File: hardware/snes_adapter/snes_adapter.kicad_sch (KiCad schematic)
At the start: 4 parts, among them J1 CART SLOT TOP ROW, J2 CART SLOT BOTTOM ROW, J3 SNES_Slot

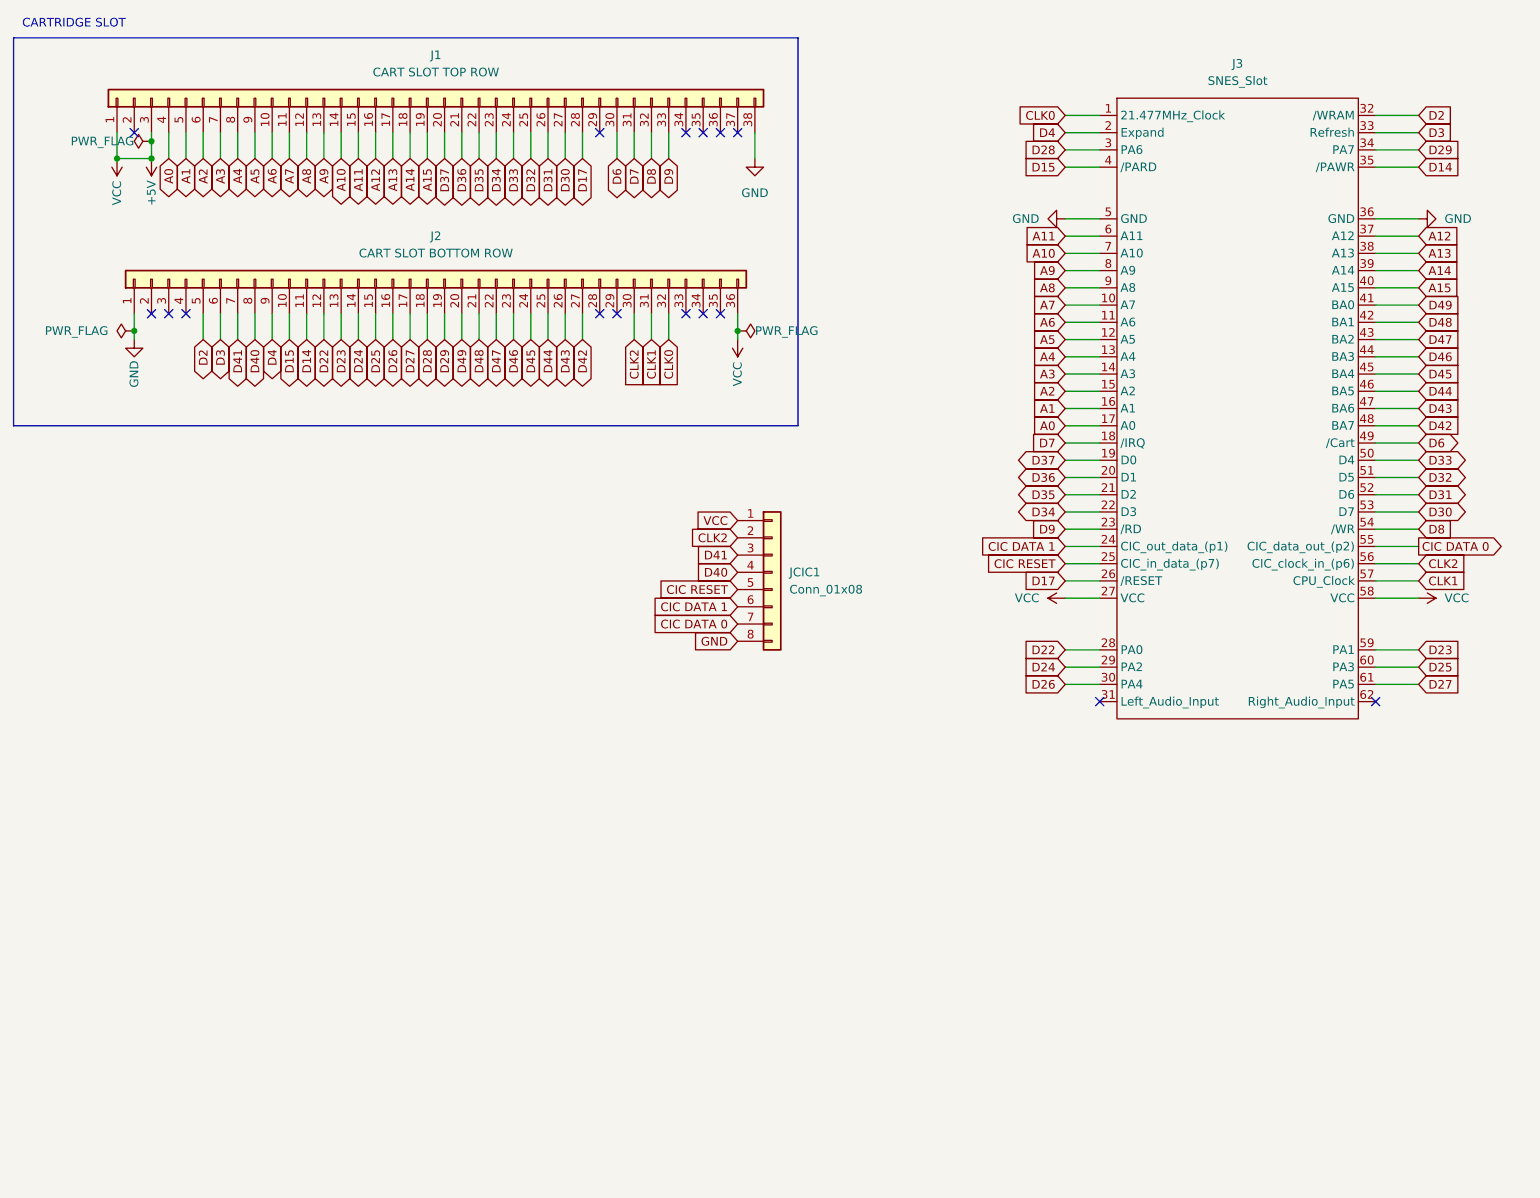
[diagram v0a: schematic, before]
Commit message: Move SNES updates to clean branch
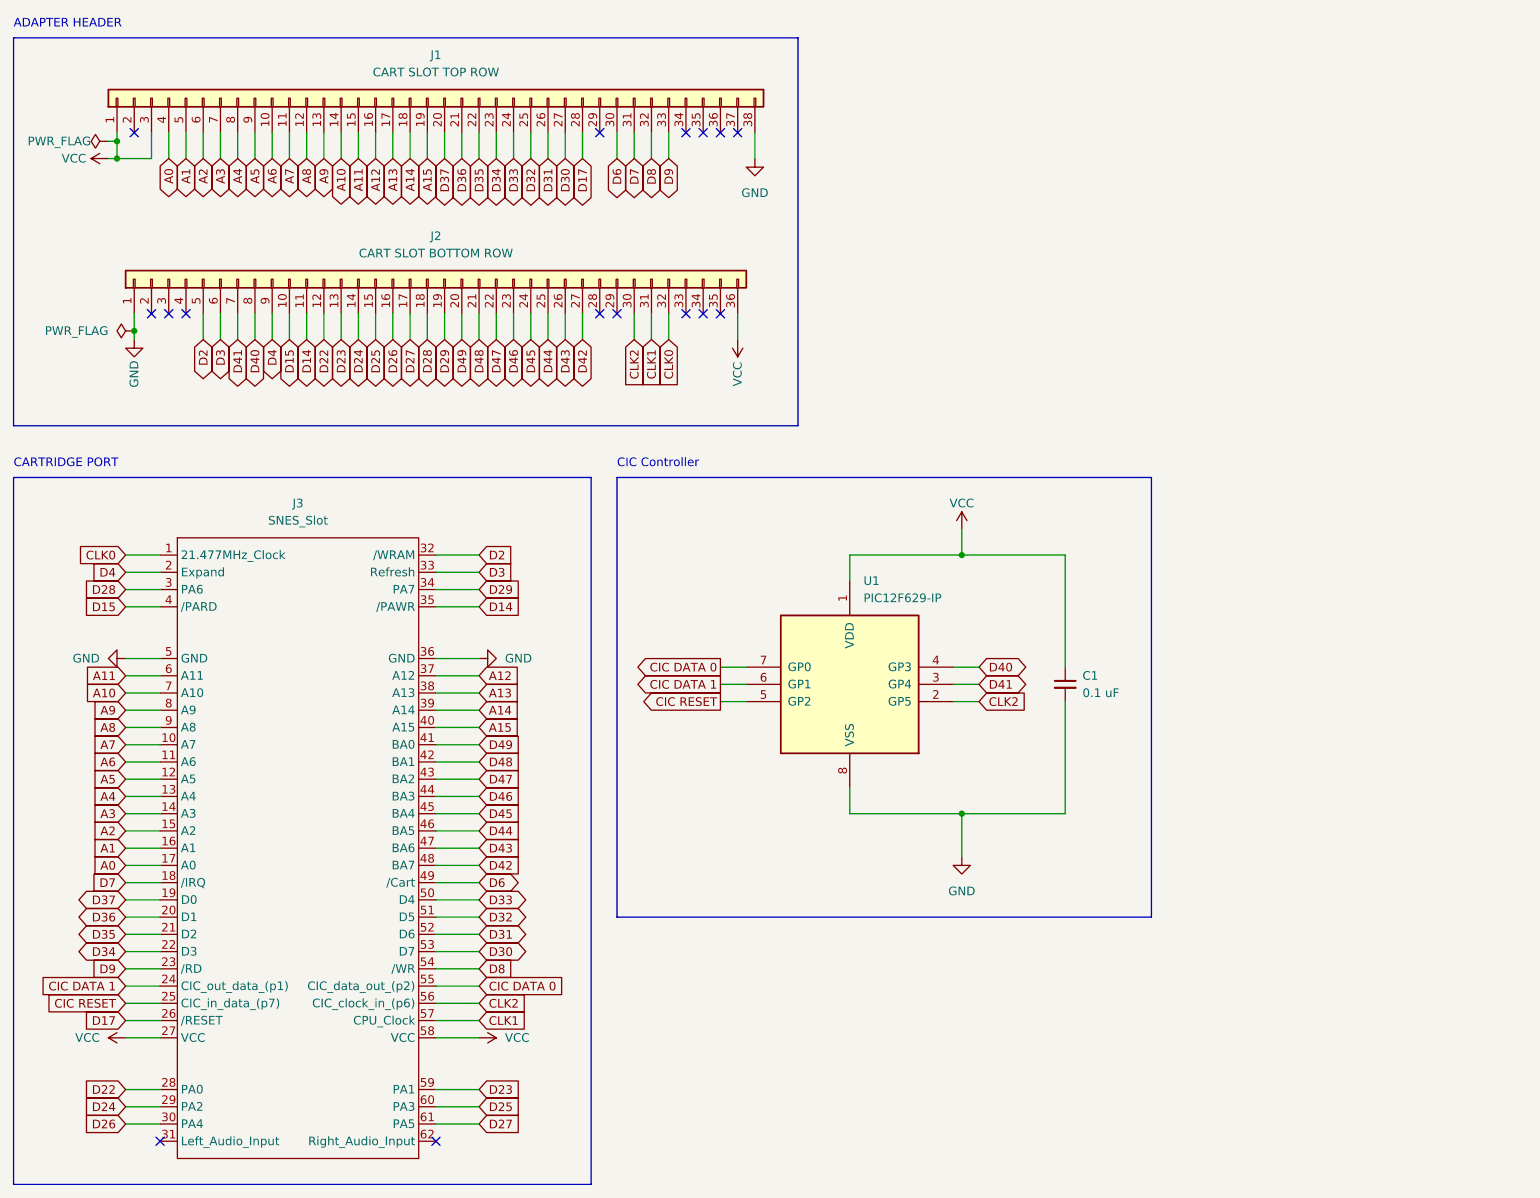
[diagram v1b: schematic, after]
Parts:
- removed JCIC1: Conn_01x08, symbol Connector_Generic:Conn_01x08
- added C1: 0.1 uF, Capacitor_THT:C_Disc_D5.0mm_W2.5mm_P5.00mm, symbol Device:C_Small
- added U1: PIC12F629-IP, Package_DIP:DIP-8_W7.62mm, symbol MCU_Microchip_PIC12:PIC12F629-IP
- J1: footprint Connector_PinSocket_2.54mm:PinSocket_1x38_P2.54mm_Vertical -> Connector_PinHeader_2.54mm:PinHeader_1x38_P2.54mm_Vertical
- J2: footprint Connector_PinSocket_2.54mm:PinSocket_1x36_P2.54mm_Vertical -> Connector_PinHeader_2.54mm:PinHeader_1x36_P2.54mm_Vertical
- J3: footprint (none) -> !OSCR:SNES Slot; symbol sanni:SNES_Slot -> !OSCR:SNES_Slot
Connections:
- net CIC DATA 0: now also U1.7 (GP0)
- net CIC DATA 1: now also U1.6 (GP1)
- net CIC RESET: now also U1.5 (GP2)
- net CLK2: now also U1.2 (GP5)
- net D40: now also U1.4 (GP3)
- net D41: now also U1.3 (GP4)
- net GND: now also C1.2, U1.8 (VSS)
- net +5V renamed VCC
- net VCC: now also C1.1, U1.1 (VDD)
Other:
- note added: "ADAPTER HEADER"
- note added: "CARTRIDGE PORT"
- note added: "CIC Controller"
- note removed: "CARTRIDGE SLOT"
- title: OSCR SNES ADAPTER -> OSCR SHIELD - SNES BREAKOUT
- moved on the sheet: J3
